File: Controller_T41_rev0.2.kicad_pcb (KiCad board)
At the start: 2 copper layers, 102.9 x 69.9 mm, 55 parts, among them J1 8P8C_x4, J2 8P8C_x4, J3 Screw_Terminal_01x02, J4 RJ45_LED, U1 Teensy4.1, U2 AMS1117-5.0, U3 74HCT245, U4 74HCT245, U5 74HCT245, U6 74HCT245

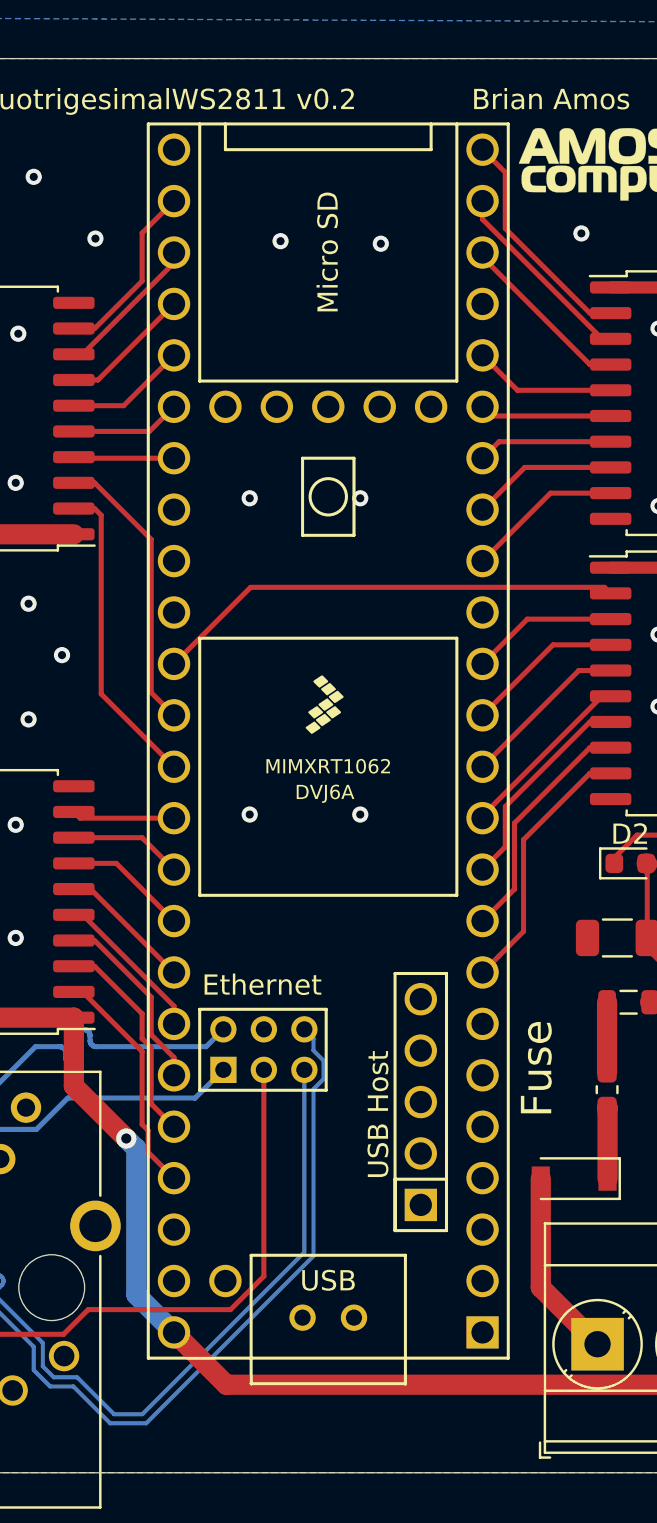
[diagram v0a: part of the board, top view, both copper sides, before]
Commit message: Added headers to 3d view
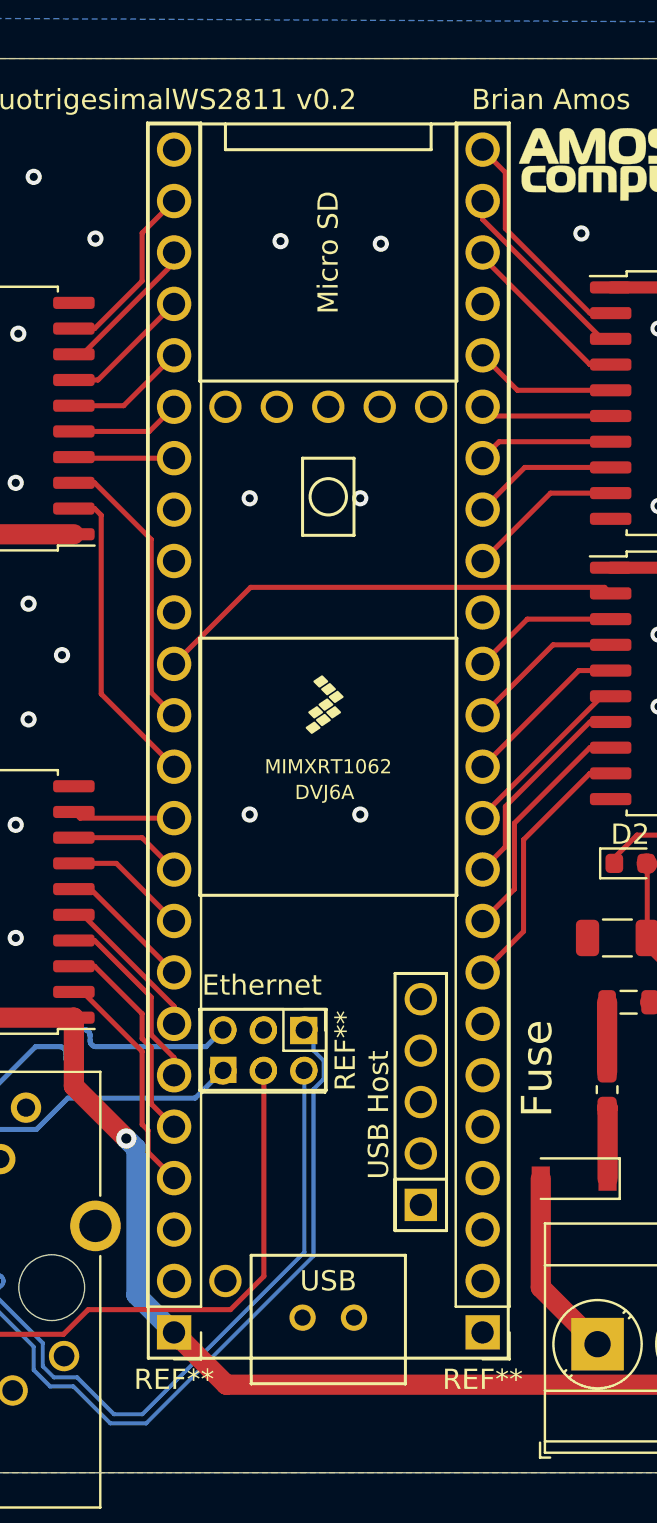
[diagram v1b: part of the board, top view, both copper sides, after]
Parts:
- added REF**: PinHeader_1x24_P2.54mm_Vertical, Connector_PinHeader_2.54mm:PinHeader_1x24_P2.54mm_Vertical, F.Cu at (141.2, 113.7)
- added REF**: PinHeader_1x24_P2.54mm_Vertical, Connector_PinHeader_2.54mm:PinHeader_1x24_P2.54mm_Vertical, F.Cu at (156.4, 113.7)
- added REF**: PinHeader_2x03_P2.00mm_Vertical, Connector_PinHeader_2.00mm:PinHeader_2x03_P2.00mm_Vertical, F.Cu at (147.6, 98.8)
